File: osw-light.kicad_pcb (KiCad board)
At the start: 4 copper layers, 36.1 x 36.1 mm, 56 parts, among them J1 Conn_02x12_Odd_Even, J2 Conn_01x06, Q1 2N7002, U1 RV-3028-C7, U2 LIS2DTW12TR, U3 ESP32-PICO-D4, U4 XC6209, U5 BQ51050BRHL, U6 XC6209

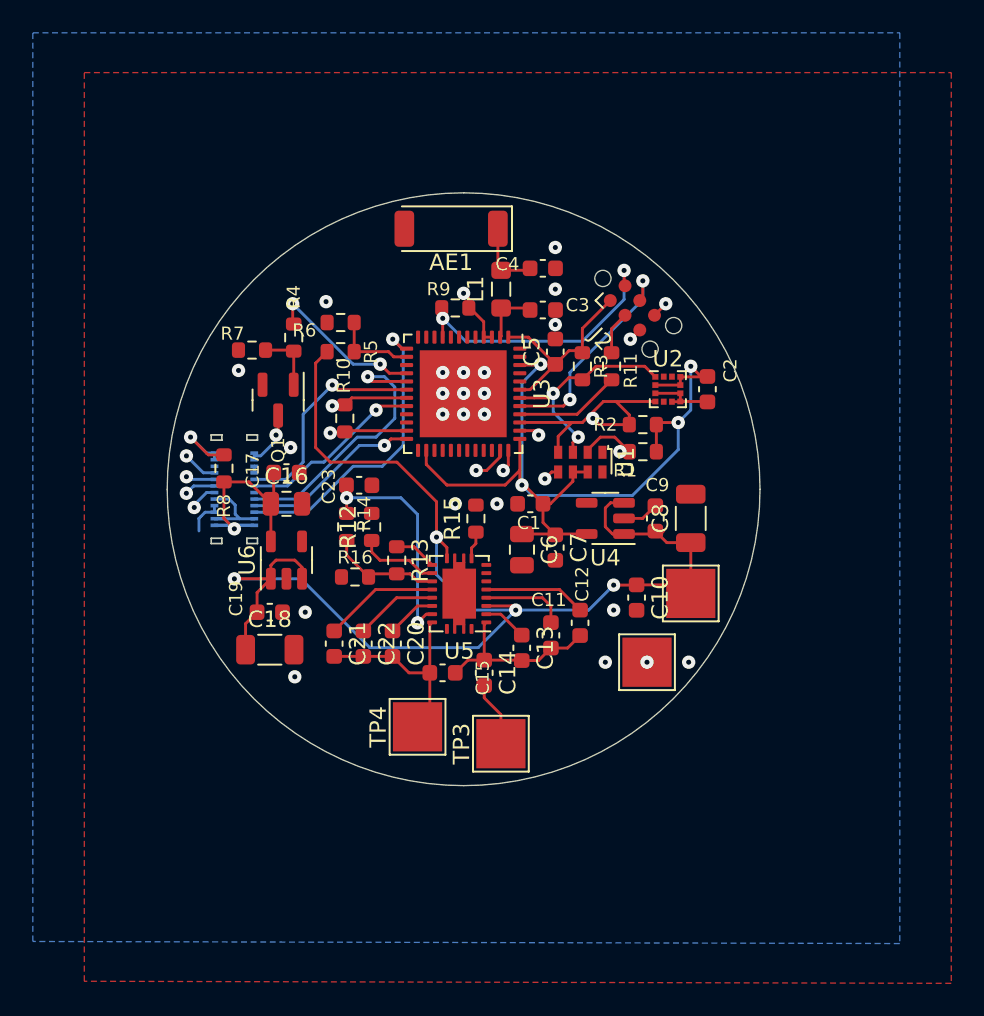
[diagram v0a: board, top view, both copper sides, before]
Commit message: Near finished with Rev2 Design
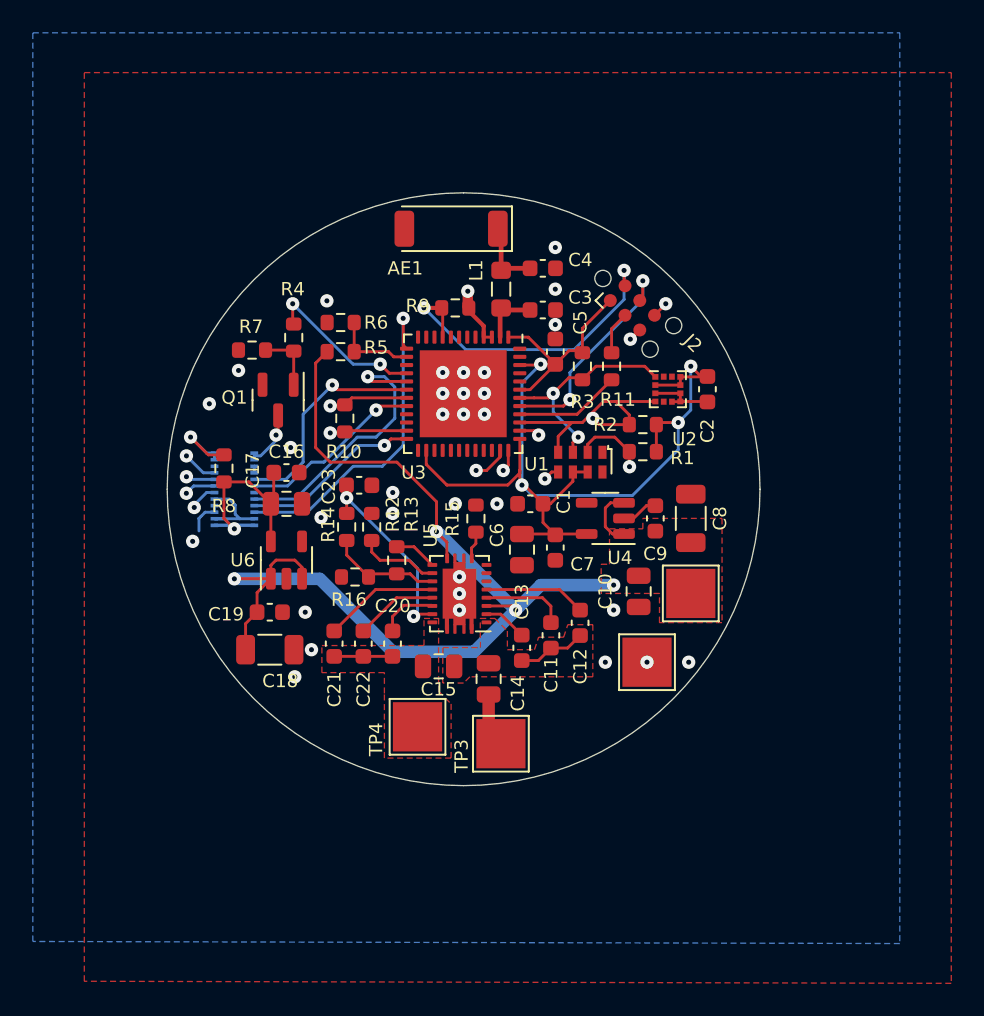
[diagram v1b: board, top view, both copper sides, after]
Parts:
- C10, C14, C15: footprint Capacitor_SMD:C_0603_1608Metric -> Capacitor_SMD:C_0805_2012Metric
- moved C15 0.46 mm to (74.7, 112.4)
- moved C14 0.45 mm to (77.7, 113.2)
- moved C10 0.40 mm to (86.9, 107.8)
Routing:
- net /VBAT: track 82.5 -> 68.6 mm
- net Net-(C15-Pad2): track 14.0 -> 3.56 mm
- net Net-(C11-Pad2): track 10.9 -> 4.19 mm
- net GND: track 11.1 -> 16.0 mm, vias 25 -> 34
- net /EN: track 17.2 -> 20.1 mm
- net Net-(C23-Pad1): track 14.2 -> 12.0 mm
- net /TFT_RST: track 18.6 -> 20.4 mm
- net +3V3: track 96.4 -> 97.2 mm
- net /RTC_INT: track 12.9 -> 13.7 mm
- net Net-(C14-Pad2): track 3.96 -> 3.31 mm
- net Net-(C20-Pad1): track 3.04 -> 3.59 mm
- added copper zone on F.Cu, net /VBAT
- added copper zone on F.Cu, net Net-(C11-Pad2)
- added copper zone on F.Cu, net Net-(C15-Pad2)
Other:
- board text added: "OpenSmartWatch E707 Light Edition Rev 2.0"
- board text removed: "OpenSmartWatch E707 Light Edition Rev 1.0"
